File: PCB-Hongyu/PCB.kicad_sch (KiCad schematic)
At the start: 25 parts, among them J2 503480-2600, Q1 BSS138, Q2 S8050, U3 AO3401

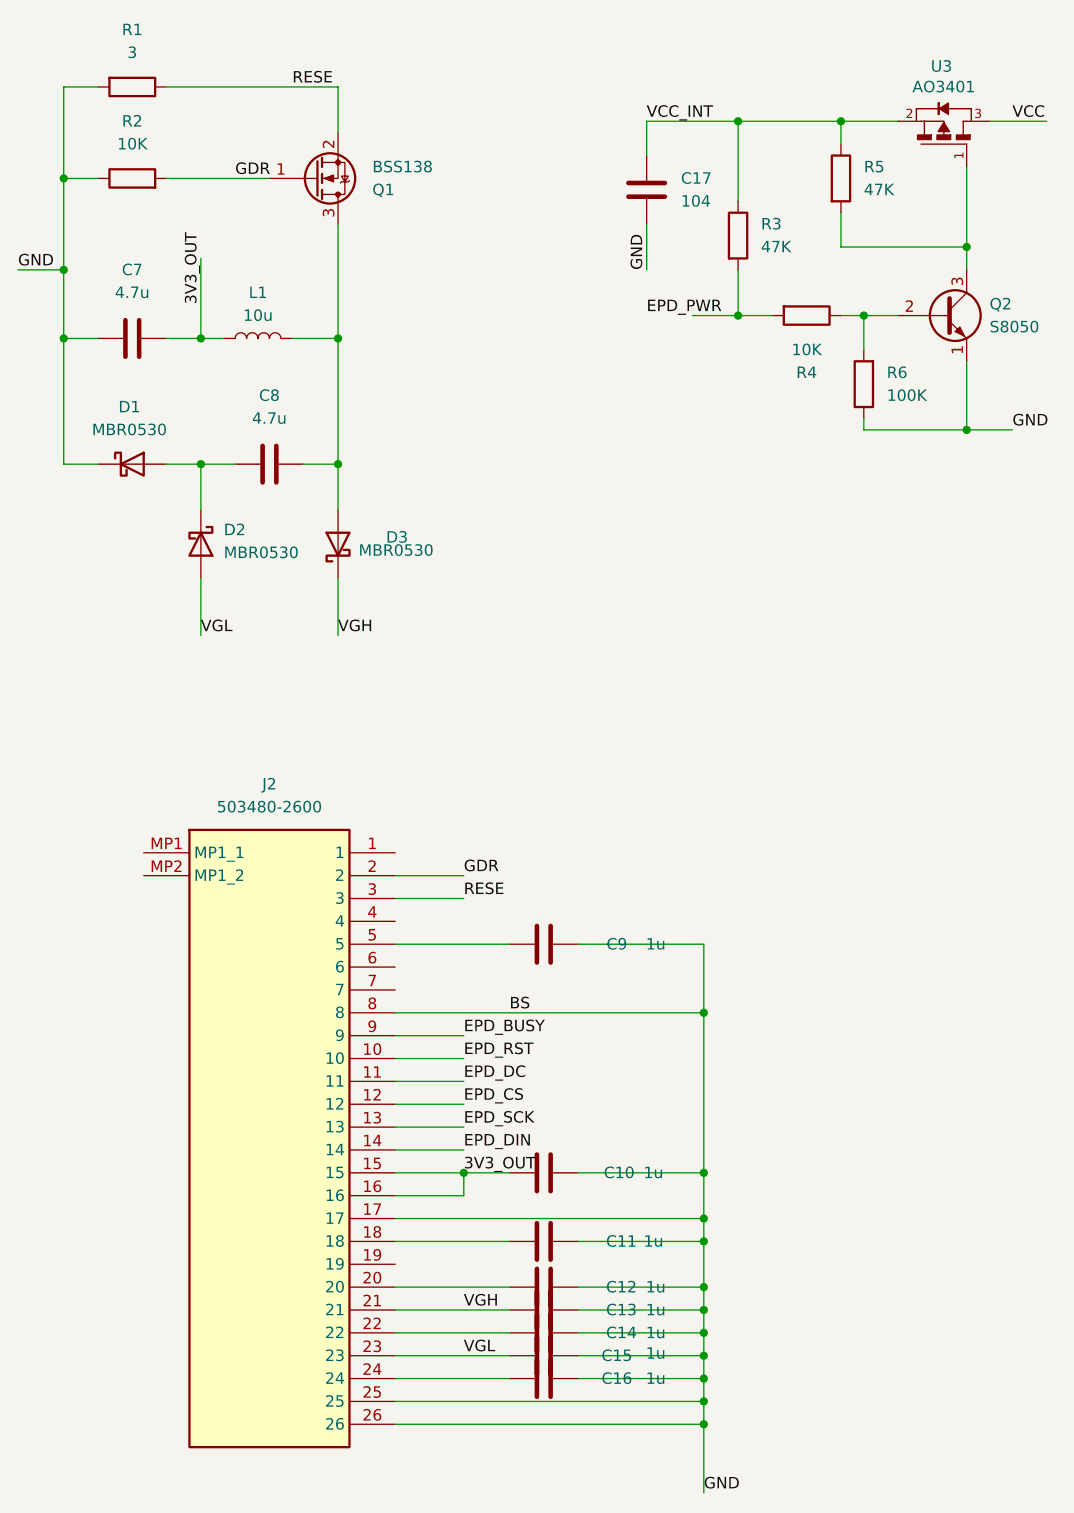
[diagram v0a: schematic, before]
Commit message: file
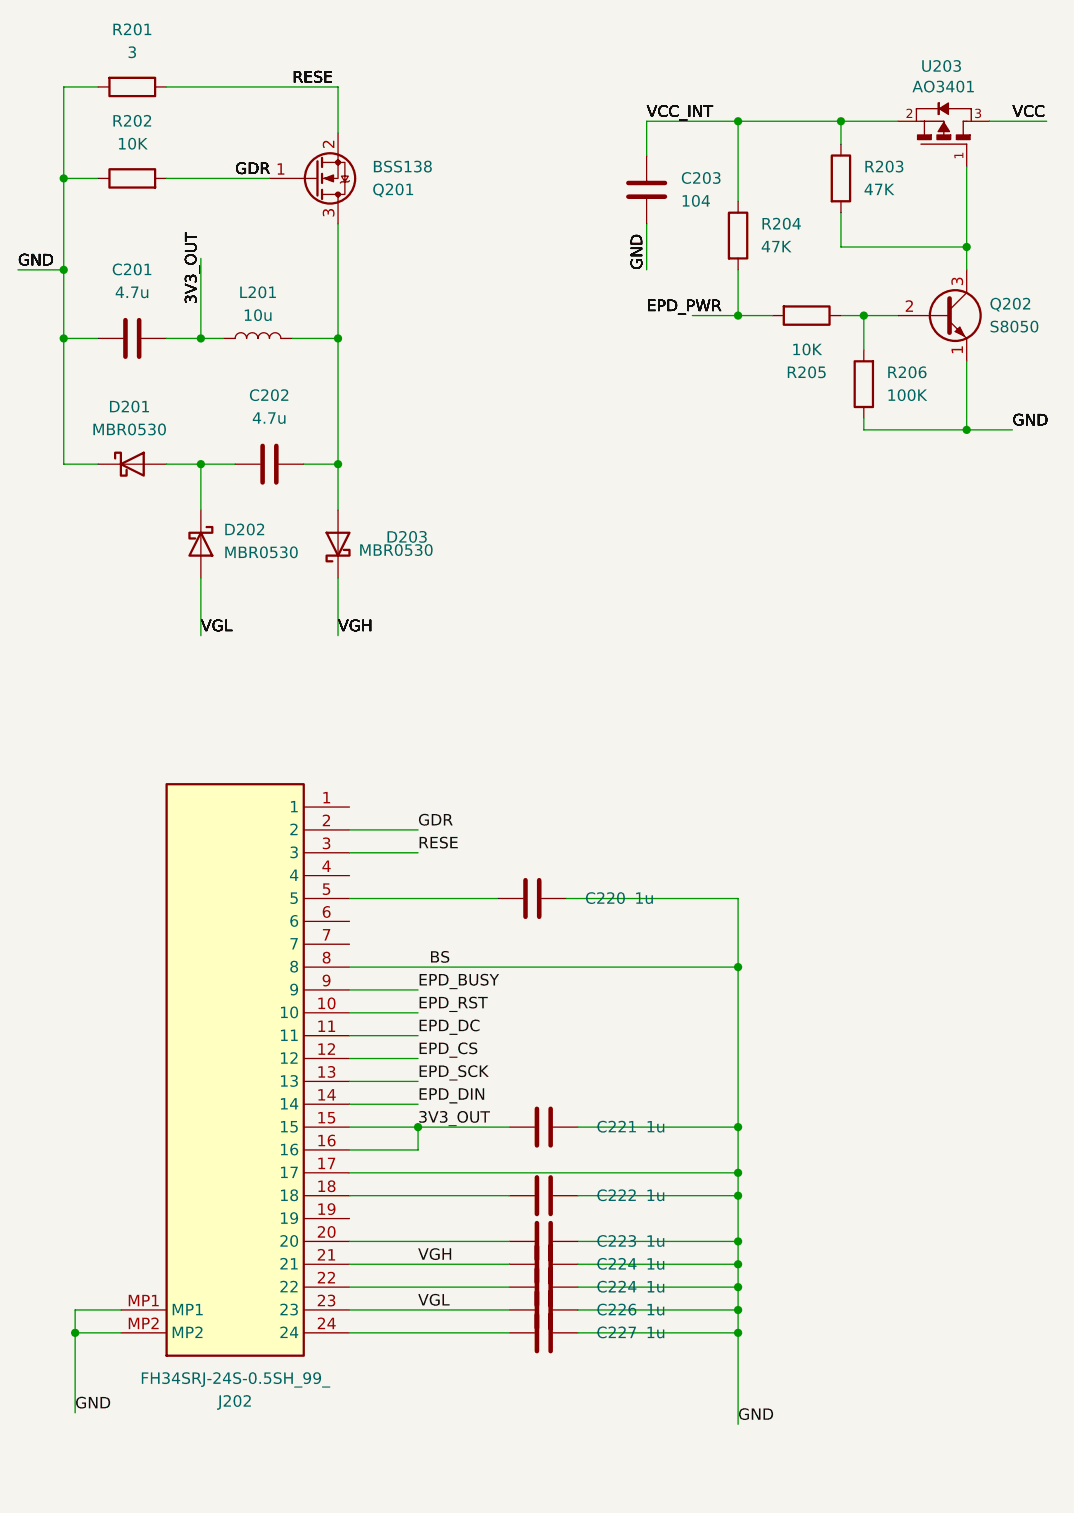
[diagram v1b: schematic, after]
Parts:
- removed C10, C11, C12, C13, C14, C15, C16, C9: 1u, Capacitor_SMD:C_0805_2012Metric_Pad1.18x1.45mm_HandSolder, symbol Device:C
- removed C17: 104, Capacitor_SMD:C_0805_2012Metric_Pad1.18x1.45mm_HandSolder, symbol Device:C
- removed C7, C8: 4.7u, Capacitor_SMD:C_0805_2012Metric_Pad1.18x1.45mm_HandSolder, symbol Device:C
- removed D1, D2: MBR0530, Diode_SMD:D_SOD-123, symbol Diode:MBR0530
- removed J2: 503480-2600, 5034802600, symbol 503480-2600:503480-2600
- removed L1: 10u, Inductor_SMD:L_0805_2012Metric_Pad1.05x1.20mm_HandSolder, symbol Device:L
- removed Q1: BSS138, Package_TO_SOT_SMD:SOT-23-3, symbol Transistor_FET:BSS138
- removed R1: 3, Resistor_SMD:R_0805_2012Metric_Pad1.20x1.40mm_HandSolder, symbol Device:R
- removed R3: 47K, Resistor_SMD:R_0805_2012Metric_Pad1.20x1.40mm_HandSolder, symbol Device:R
- removed R4: 10K, Resistor_SMD:R_0805_2012Metric_Pad1.20x1.40mm_HandSolder, symbol Device:R
- removed R6: 100K, Resistor_SMD:R_0805_2012Metric_Pad1.20x1.40mm_HandSolder, symbol Device:R
- removed U3: AO3401, Custom:SOT23, symbol AO3401:AO3401
- added C201, C202: 4.7u, Capacitor_SMD:C_0805_2012Metric_Pad1.18x1.45mm_HandSolder, symbol Device:C
- added C203: 104, Capacitor_SMD:C_0805_2012Metric_Pad1.18x1.45mm_HandSolder, symbol Device:C
- added C220, C221, C222, C223, C224 (x2), C226, C227: 1u, Capacitor_SMD:C_0805_2012Metric_Pad1.18x1.45mm_HandSolder, symbol Device:C
- added D201, D202: MBR0530, Diode_SMD:D_SOD-123, symbol Diode:MBR0530
- added J202: FH34SRJ-24S-0.5SH_99_, Custom:FH34SRJ24S05SH99, symbol FH34SRJ-24S-0.5SH(99):FH34SRJ-24S-0.5SH_99_
- added L201: 10u, Inductor_SMD:L_0805_2012Metric_Pad1.05x1.20mm_HandSolder, symbol Device:L
- added Q201: BSS138, Package_TO_SOT_SMD:SOT-23-3, symbol Transistor_FET:BSS138
- added R201: 3, Resistor_SMD:R_0805_2012Metric_Pad1.20x1.40mm_HandSolder, symbol Device:R
- added R204: 47K, Resistor_SMD:R_0805_2012Metric_Pad1.20x1.40mm_HandSolder, symbol Device:R
- added R205: 10K, Resistor_SMD:R_0805_2012Metric_Pad1.20x1.40mm_HandSolder, symbol Device:R
- added R206: 100K, Resistor_SMD:R_0805_2012Metric_Pad1.20x1.40mm_HandSolder, symbol Device:R
- added U203: AO3401, Custom:SOT23, symbol AO3401:AO3401
- Q202: renamed from Q2; footprint Package_TO_SOT_SMD:SOT-23-3 -> Package_TO_SOT_THT:TO-92_Inline
- renumbered D3 to D203, R2 to R202, R5 to R203
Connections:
- net 3V3_OUT: now also C201.2, C221.1, J202.15, J202.16, L201.1
- net BS: now also C201.1, C203.2, C220.2, C221.2, C222.2, C223.2, C224.2, C224.2, C226.2, C227.2, D201.1 (K), J202.17, J202.8, J202.MP1, J202.MP2, R201.2, R206.1
- net EPD_BUSY: now also J202.9
- net EPD_CS: now also J202.12
- net EPD_DC: now also J202.11
- net EPD_DIN: now also J202.14
- net EPD_RST: now also J202.10
- net EPD_SCK: now also J202.13
- net GDR: now also J202.2, Q201.1 (G)
- net RESE: now also J202.3, Q201.2 (S), R201.1
- net VCC: now also U203.3
- net VCC_INT: now also C203.1, R204.1, U203.2
- net VGH: now also C224.1, J202.21
- net VGL: now also C226.1, D202.2 (A), J202.23
- net at D203.2 (A): now also C202.2, L201.2, Q201.3 (D)
- net at Q202.3 (C), R203.2: now also U203.1
- net at Q202.2 (B): now also R205.1, R206.2
- new net: C222.1, J202.18
- new net: C223.1, J202.20
- new net: C224.1, J202.22
- new net: C227.1, J202.24
- new net: C220.1, J202.5
- new net: C202.1, D201.2 (A), D202.1 (K)
- new net: R204.2, R205.2
